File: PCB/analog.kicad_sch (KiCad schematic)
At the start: 0 parts

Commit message: Firmware dump and PCB update
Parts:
- added C10, C12: 220p, cipulot_parts:C_0603_1608Metric_Pad1.08x0.95mm_HandSolder, symbol Device:C
- added C11, C9: 0.1u, cipulot_parts:C_0603_1608Metric_Pad1.08x0.95mm_HandSolder, symbol Device:C
- added R10, R11, R12, R13, R14, R15, R16, R17, R18, R19, R20, R21, R22, R23, R24, R9: 100k, cipulot_parts:R_0603_1608Metric_Pad0.98x0.95mm_HandSolder, symbol Device:R
- added U2, U3: 74HC4051, cipulot_parts:TSSOP16, symbol 74xx:74HC4051
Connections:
- new net CHARGE_RST: C10.1, C12.1, U2.3 (A), U3.3 (A)
- new net COL0: R15.1, U2.2 (A6)
- new net COL1: R13.1, U2.1 (A4)
- new net COL10: R20.1, U3.12 (A3)
- new net COL11: R17.1, U3.13 (A0)
- new net COL12: R18.1, U3.14 (A1)
- new net COL13: R19.1, U3.15 (A2)
- new net COL14: R22.1, U3.5 (A5)
- new net COL15: R24.1, U3.4 (A7)
- new net COL2: R12.1, U2.12 (A3)
- new net COL3: R9.1, U2.13 (A0)
- new net COL4: R10.1, U2.14 (A1)
- new net COL5: R11.1, U2.15 (A2)
- new net COL6: R14.1, U2.5 (A5)
- new net COL7: R16.1, U2.4 (A7)
- new net COL8: R23.1, U3.2 (A6)
- new net COL9: R21.1, U3.1 (A4)
- new net COL_EN: U2.6 (~{E}), U3.6 (~{E})
- new net CSEL0: U2.11 (S0), U3.11 (S0)
- new net CSEL1: U2.10 (S1), U3.10 (S1)
- new net CSEL2: U2.9 (S2), U3.9 (S2)
- new net GND: C10.2, C11.1, C12.2, C9.1, R10.2, R11.2, R12.2, R13.2, R14.2, R15.2, R16.2, R17.2, R18.2, R19.2, R20.2, R21.2, R22.2, R23.2, R24.2, R9.2, U2.7 (VEE), U2.8 (GND), U3.7 (VEE), U3.8 (GND)
- new net VCC: C11.2, C9.2, U2.16 (VCC), U3.16 (VCC)

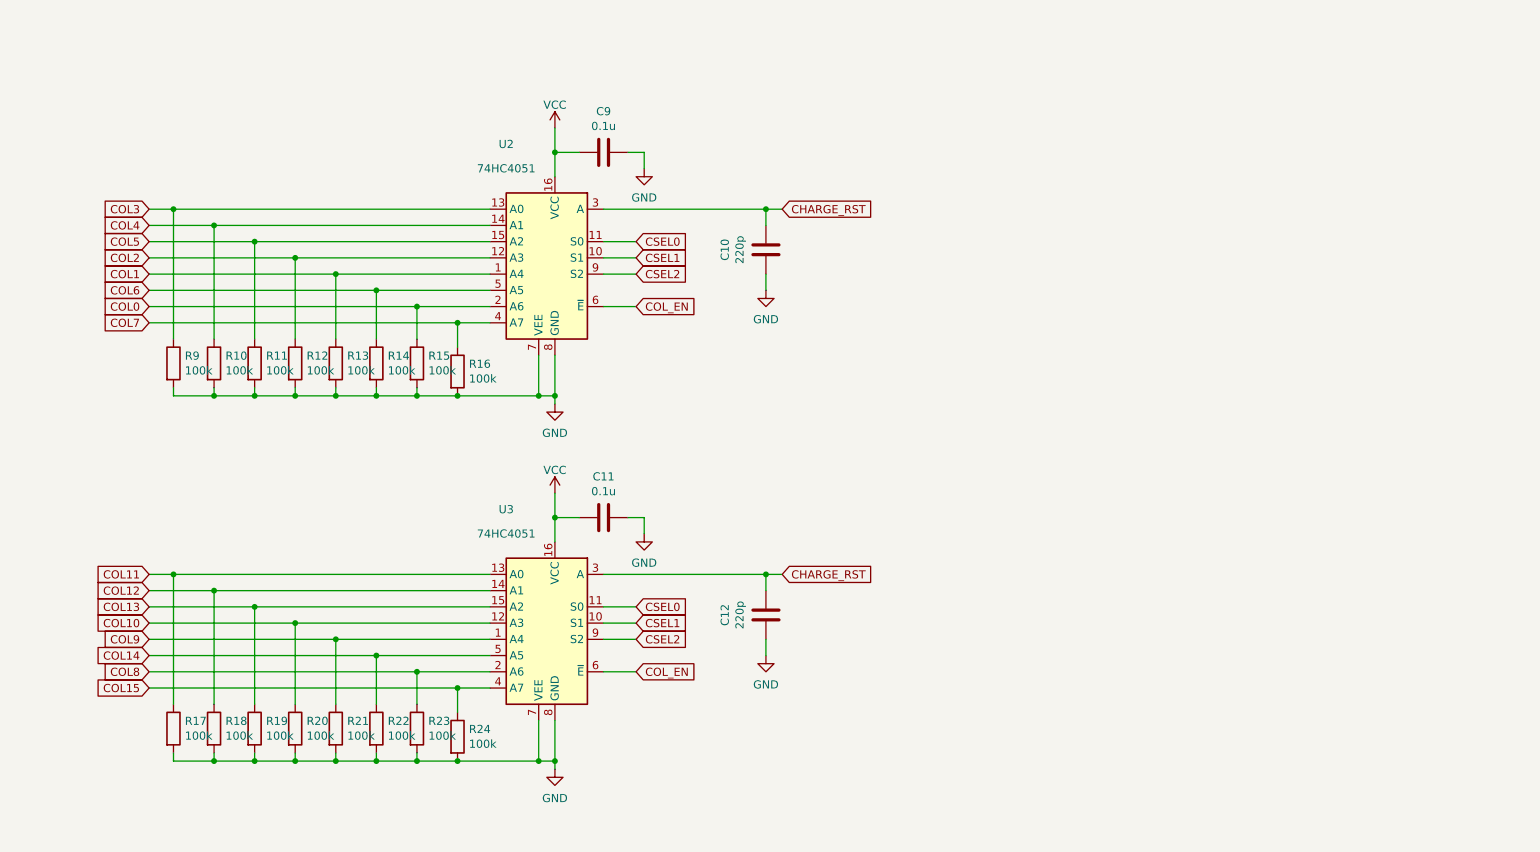
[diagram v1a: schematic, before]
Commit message: Update
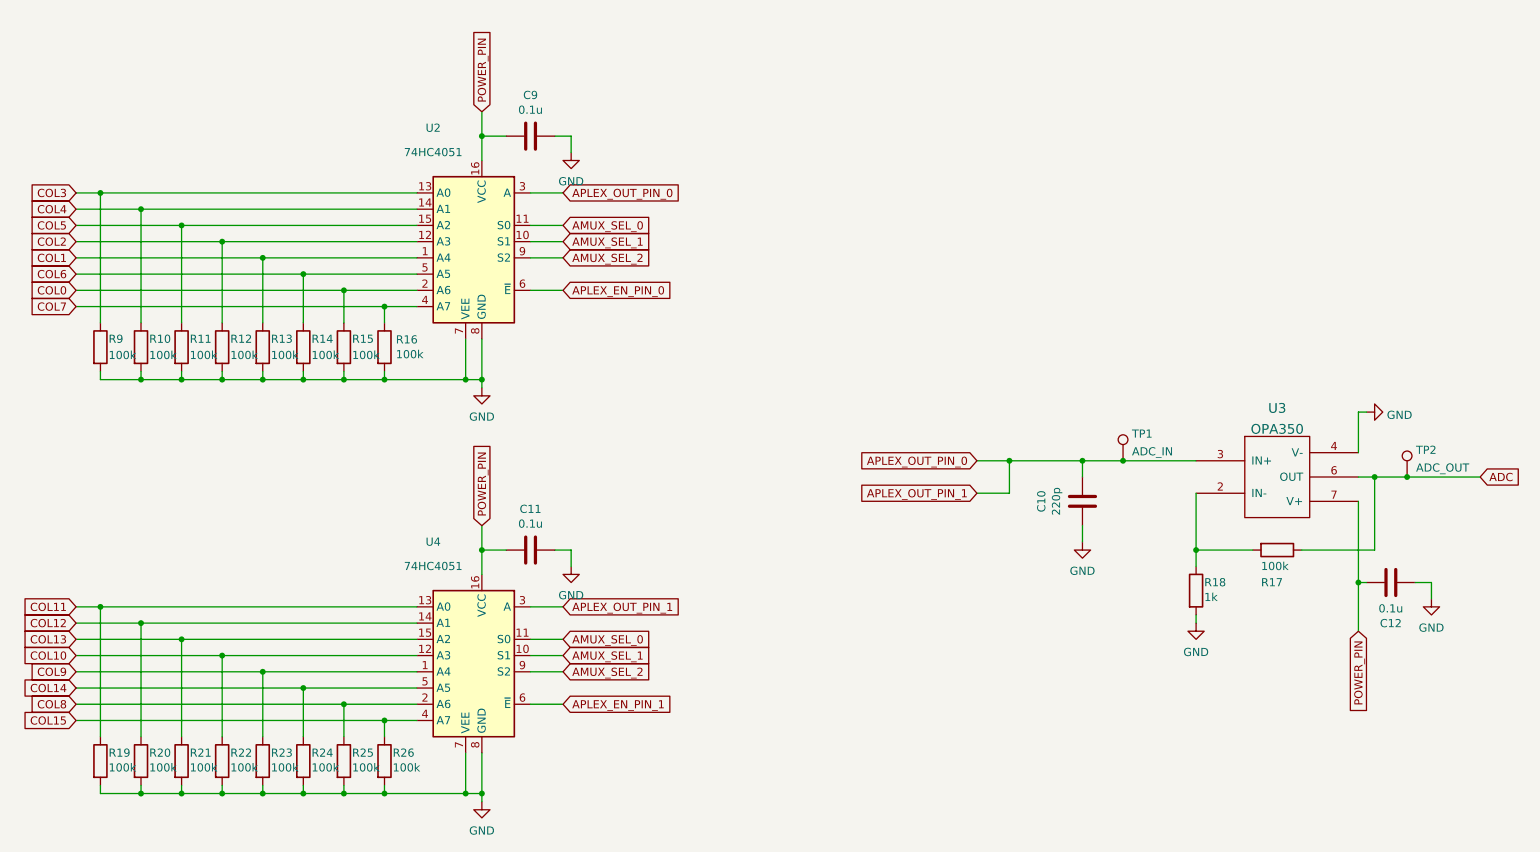
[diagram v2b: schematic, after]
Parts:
- added R17: 100k, Resistor_SMD:R_0603_1608Metric, symbol Device:R
- added R18: 1k, Resistor_SMD:R_0603_1608Metric, symbol Device:R
- added TP1: ADC_IN, TestPoint:TestPoint_Pad_D1.0mm, symbol Connector:TestPoint
- added TP2: ADC_OUT, TestPoint:TestPoint_Pad_D1.0mm, symbol Connector:TestPoint
- added U3: OPA350, Package_SO:SOIC-8_3.9x4.9mm_P1.27mm, symbol burrbrown:OPA350
- C10, C11, C9: footprint cipulot_parts:C_0603_1608Metric_Pad1.08x0.95mm_HandSolder -> Capacitor_SMD:C_0603_1608Metric
- C12: value 220p -> 0.1u; footprint cipulot_parts:C_0603_1608Metric_Pad1.08x0.95mm_HandSolder -> Capacitor_SMD:C_0603_1608Metric
- R10, R11, R12, R13, R14, R15, R16, R9: footprint cipulot_parts:R_0603_1608Metric_Pad0.98x0.95mm_HandSolder -> Resistor_SMD:R_0603_1608Metric
- R19: renamed from R17; footprint cipulot_parts:R_0603_1608Metric_Pad0.98x0.95mm_HandSolder -> Resistor_SMD:R_0603_1608Metric
- R20: renamed from R18; footprint cipulot_parts:R_0603_1608Metric_Pad0.98x0.95mm_HandSolder -> Resistor_SMD:R_0603_1608Metric
- R21: renamed from R19; footprint cipulot_parts:R_0603_1608Metric_Pad0.98x0.95mm_HandSolder -> Resistor_SMD:R_0603_1608Metric
- R22: renamed from R20; footprint cipulot_parts:R_0603_1608Metric_Pad0.98x0.95mm_HandSolder -> Resistor_SMD:R_0603_1608Metric
- R23: renamed from R21; footprint cipulot_parts:R_0603_1608Metric_Pad0.98x0.95mm_HandSolder -> Resistor_SMD:R_0603_1608Metric
- R24: renamed from R22; footprint cipulot_parts:R_0603_1608Metric_Pad0.98x0.95mm_HandSolder -> Resistor_SMD:R_0603_1608Metric
- R25: renamed from R23; footprint cipulot_parts:R_0603_1608Metric_Pad0.98x0.95mm_HandSolder -> Resistor_SMD:R_0603_1608Metric
- R26: renamed from R24; footprint cipulot_parts:R_0603_1608Metric_Pad0.98x0.95mm_HandSolder -> Resistor_SMD:R_0603_1608Metric
- renumbered U3 to U4
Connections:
- net GND: now also C12.1, R18.2, U3.4 (V-); no longer C12.2
- net CHARGE_RST renamed APLEX_OUT_PIN_0
- net APLEX_OUT_PIN_0: now also TP1.1, U3.3 (IN+); no longer C12.1
- net COL_EN renamed APLEX_EN_PIN_0
- net APLEX_EN_PIN_0: no longer U4.6 (~{E})
- net CSEL0 renamed AMUX_SEL_0
- net CSEL1 renamed AMUX_SEL_1
- net CSEL2 renamed AMUX_SEL_2
- net VCC renamed POWER_PIN
- net POWER_PIN: now also C12.2, U3.7 (V+)
- new net: R17.2, R18.1, U3.2 (IN-)
- new net ADC: R17.1, TP2.1, U3.6 (OUT)
- new net APLEX_EN_PIN_1: U4.6 (~{E})
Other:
- moved on the sheet: C10, C11, C9, R10, R11, R12, R13, R14, R15, R16, R19, R20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
